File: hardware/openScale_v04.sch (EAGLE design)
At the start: 72 parts, among them J1 3.3V, J2 UL, J3 UR, J4 LL, J5 LR, Q1 200mA/50V, Q2 200mA/50V, Q3 MMBT4403, Q4 MOSFET-NCHANNEL2N7002PW, U1 HX711, U3 TMP102, U4 ATMEGA328P_TQFP, U6 FT231XS, Y2 16MHZ

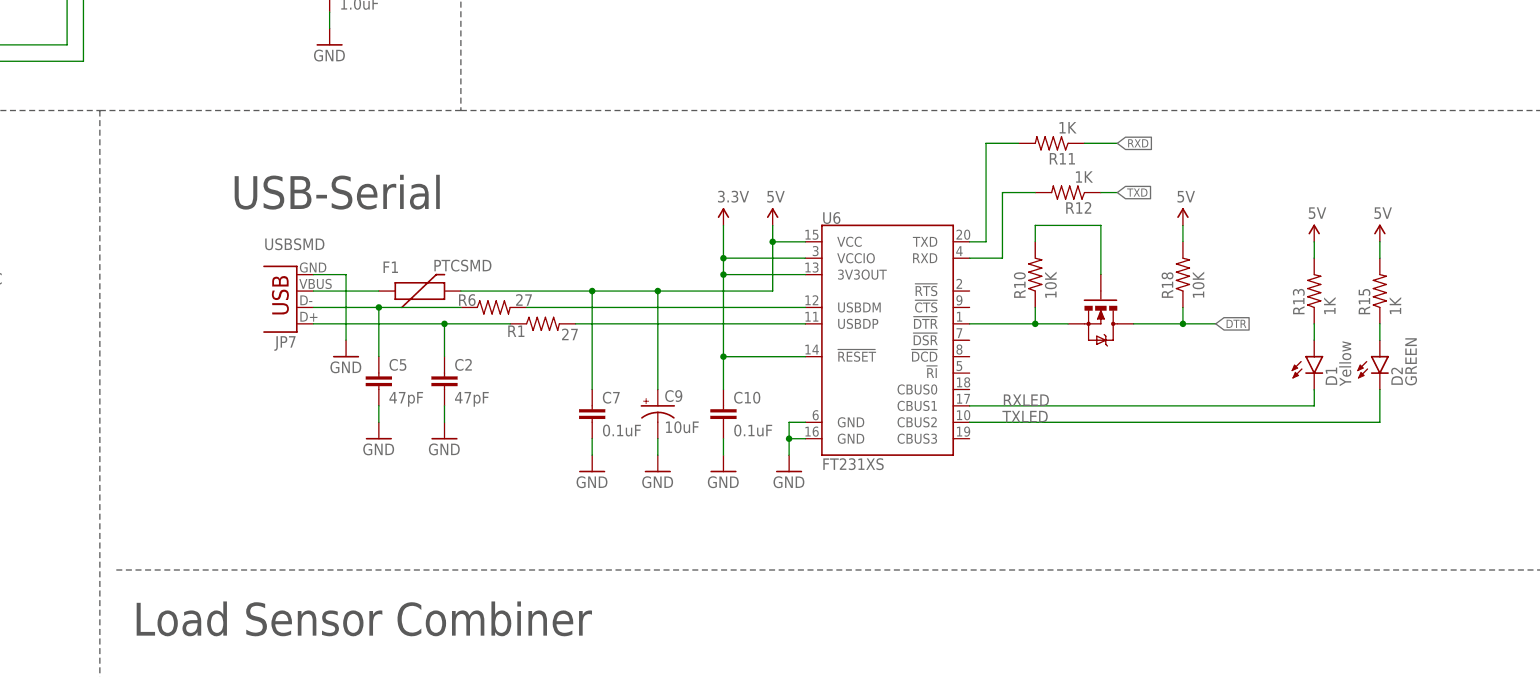
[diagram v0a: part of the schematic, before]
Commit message: Updated Board and Schemtic
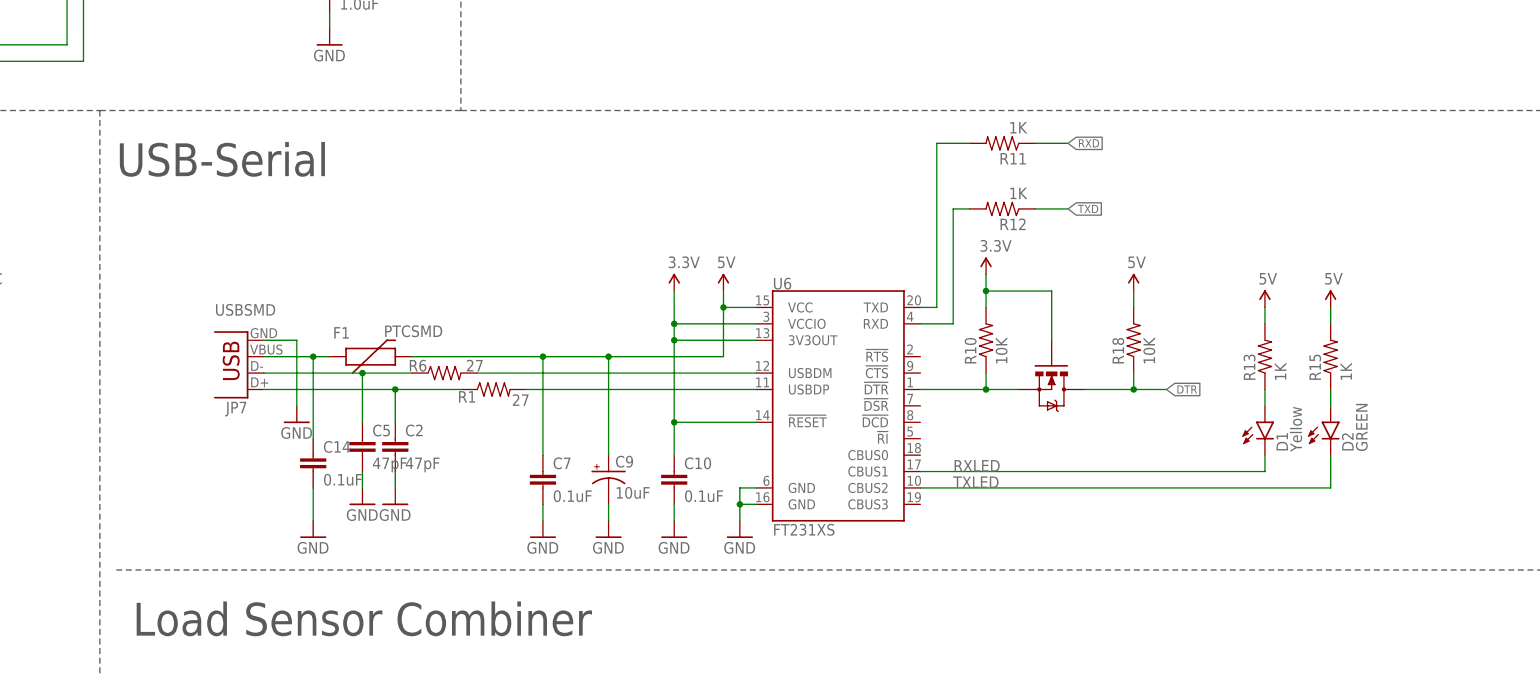
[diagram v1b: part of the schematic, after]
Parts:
- added C14: 0.1uF, SparkFun-Capacitors:0.1UF-25V(+80/-20%)(0603)
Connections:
- removed net N$33: Q4.G, R10.2
- net 3.3V: now also Q4.G, R10.2
- net GND: now also C14.2
- net N$12: now also C14.1
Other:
- moved on the sheet: C10, C2, C5, C7, C9, D1, D2, F1, JP7, R1, R10, R11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
